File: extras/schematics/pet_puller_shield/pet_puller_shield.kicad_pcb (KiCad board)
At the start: 2 copper layers, 16 parts, among them J1 Jack-DC, J2 Conn_01x02, J3 Conn_01x02, J4 Conn_01x02, J5 Conn_01x04, Q1 IRF540N, U1 LM317_TO-220, U2 MX1508_module

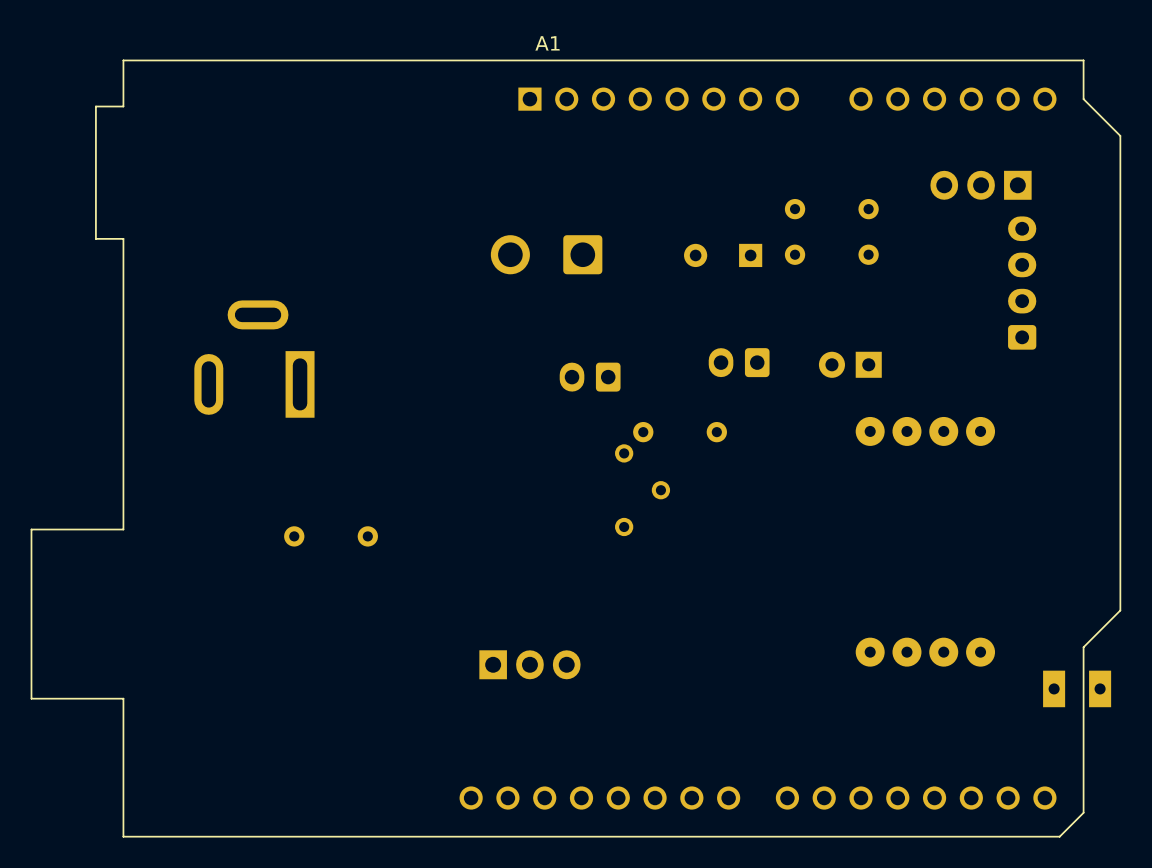
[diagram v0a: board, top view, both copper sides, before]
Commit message: Updated schematics
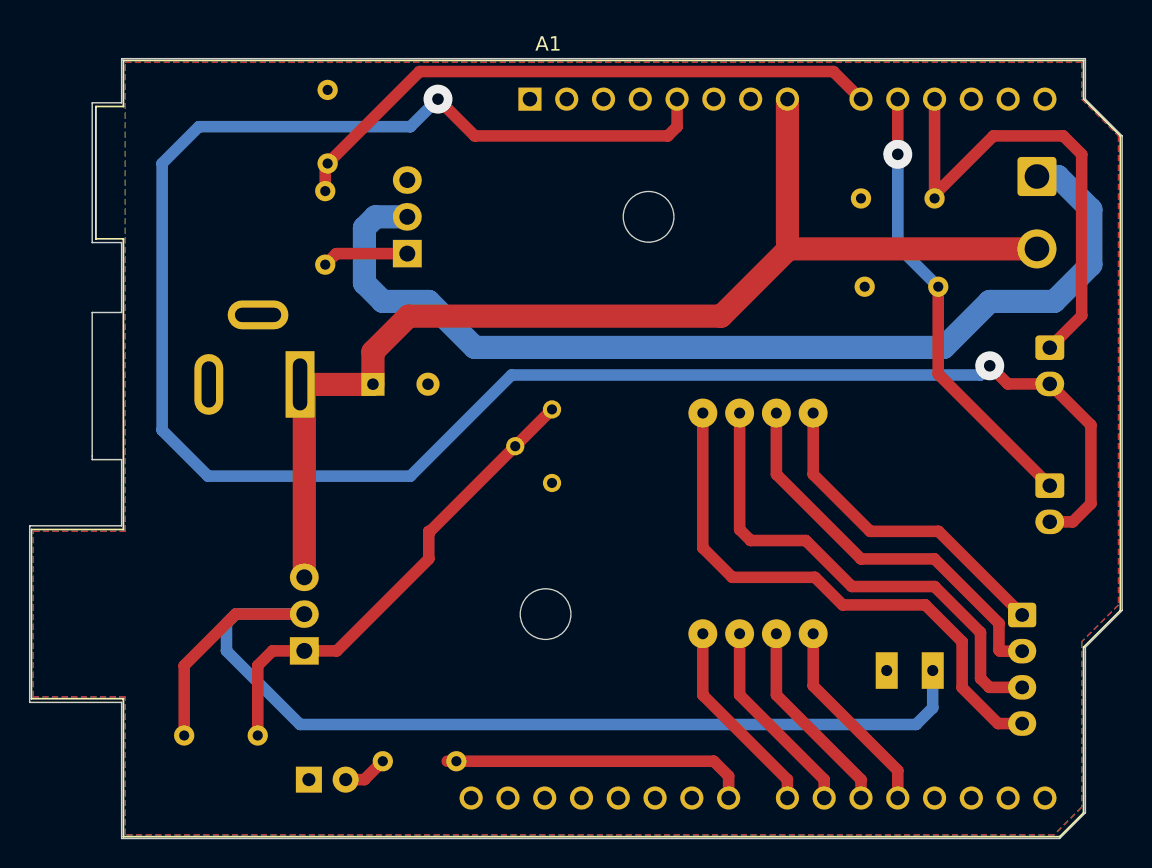
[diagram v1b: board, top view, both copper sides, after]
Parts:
- added R5: 10k, Resistor_THT:R_Axial_DIN0204_L3.6mm_D1.6mm_P5.08mm_Horizontal, B.Cu at (137.2, 89.5)
- added R6: 220, Resistor_THT:R_Axial_DIN0204_L3.6mm_D1.6mm_P5.08mm_Horizontal, B.Cu at (137.0, 96.5)
- Q1, U1: footprint Package_TO_SOT_THT:TO-220-3_Vertical -> Package_TO_SOT_THT:TO-220-3_Horizontal_TabDown
- moved U1 58.8 mm to (135.6, 123.2), turned to 90 degrees
- moved D1 48.1 mm to (135.9, 132.1), turned to 0 degrees
- moved J4 31.8 mm to (186.1, 90.4), turned to -90 degrees
- moved J3 30.6 mm to (187.0, 102.3), turned to -90 degrees
- moved Q1 29.0 mm to (142.7, 95.8), turned to 90 degrees
- moved R2 29.0 mm to (146.1, 130.8)
- moved C1 27.6 mm to (140.3, 104.8), turned to 0 degrees
- moved J2 21.9 mm to (187.0, 111.8), turned to -90 degrees
- moved J5 19.2 mm to (185.1, 120.7), turned to -90 degrees
- moved R4 15.7 mm to (132.3, 129.0)
- moved U2 11.6 mm to (174.5, 99.8)
- moved RV1 9.53 mm to (152.7, 106.5), turned to 0 degrees
- moved R1 5.37 mm to (174.2, 98.0), turned to 0 degrees
- moved R3 3.92 mm to (174.0, 91.9), turned to 0 degrees
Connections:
- A1 pad 10: unconnected-(A1-Pad10) -> RUNOUT
- A1 pad 11: unconnected-(A1-Pad11) -> THERMISTOR
- A1 pad 17: M0 -> unconnected-(A1-Pad17)
- A1 pad 18: M1 -> unconnected-(A1-Pad18)
- A1 pad 19: M2 -> M0
- A1 pad 20: M3 -> M1
- A1 pad 21: HOTEND -> M2
- A1 pad 22: RUNOUT -> M3
- A1 pad 9: THERMISTOR -> HOTEND
- Q1 pad 1: HOTEND -> Net-(Q1-Pad1)
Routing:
- net +5V: track 0.00 -> 138.1 mm, vias 0 -> 2
- net +12V: track 0.00 -> 79.9 mm
- net +9V: track 0.00 -> 76.1 mm
- net Net-(J4-Pad1): track 0.00 -> 69.9 mm
- net HOTEND: track 0.00 -> 42.2 mm
- net Net-(J5-Pad4): track 0.00 -> 38.2 mm
- net Net-(J5-Pad3): track 0.00 -> 33.9 mm
- net THERMISTOR: track 0.00 -> 33.6 mm
- net Net-(R4-Pad1): track 0.00 -> 33.6 mm
- net RUNOUT: track 0.00 -> 31.0 mm, vias 0 -> 1
- net Net-(J5-Pad2): track 0.00 -> 27.3 mm
- net Net-(J5-Pad1): track 0.00 -> 22.7 mm
- net LED: track 0.00 -> 21.4 mm
- net M0: track 0.00 -> 13.8 mm
- net M1: track 0.00 -> 13.8 mm
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- added copper zone on B.Cu, net GND
- added copper zone on F.Cu, net GND
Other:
- board outline added: 75.4 x 53.8 mm
